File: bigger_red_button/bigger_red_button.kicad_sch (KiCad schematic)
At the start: 22 parts, among them J1 USB_C_Receptacle_USB2.0_16P, J2 Conn_02x05_Odd_Even, J3 Conn_02x01, J4 Conn_02x01, U1 USBLC6-2SC6, U2 TPS7A0533PDBV, U3 STM32C071FBPx, U4 PAM2804

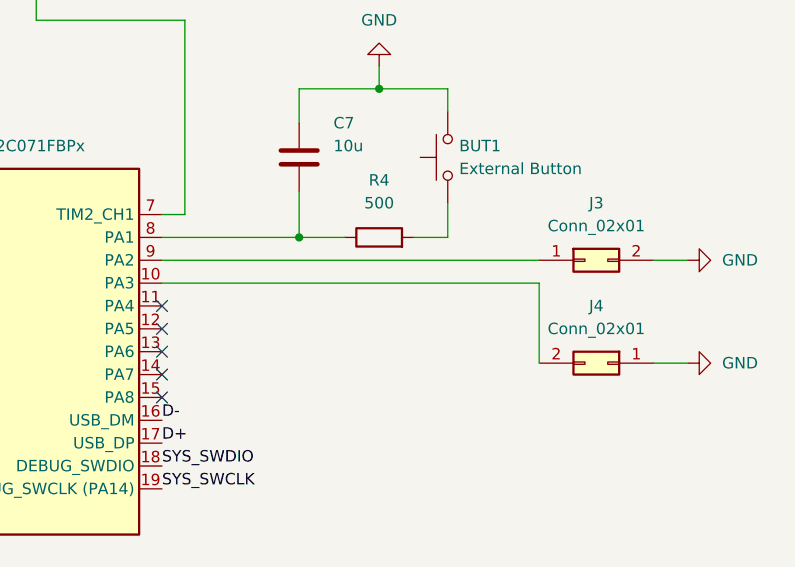
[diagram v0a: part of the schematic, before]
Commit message: Replace jumper symbols
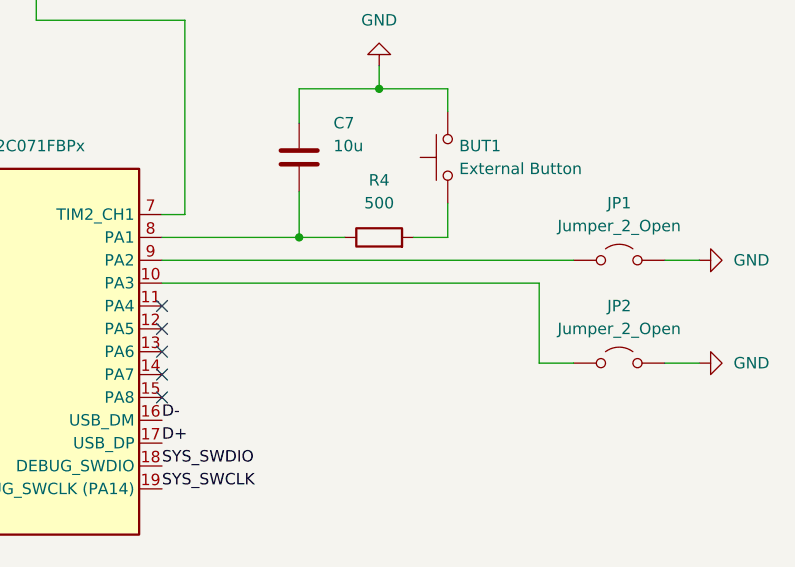
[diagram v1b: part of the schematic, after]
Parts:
- removed J3, J4: Conn_02x01, Connector_PinHeader_2.54mm:PinHeader_1x02_P2.54mm_Vertical, symbol Connector_Generic:Conn_02x01
- added JP1, JP2: Jumper_2_Open, Connector_PinHeader_2.54mm:PinHeader_1x02_P2.54mm_Vertical, symbol Jumper:Jumper_2_Open
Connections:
- net GND: now also JP1.2 (B), JP2.2 (B)
- net at U3.10 (PA3): now also JP2.1 (A)
- net at U3.9 (PA2): now also JP1.1 (A)
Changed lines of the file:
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@@
 	(wire
 		(pts
-			(xy 252.73 106.68) (xy 256.54 106.68)
+			(xy 254 106.68) (xy 257.81 106.68)
 		)
 		(stroke
@@
 	(wire
 		(pts
+			(xy 240.03 118.11) (xy 243.84 118.11)
+		)
+		(stroke
+			(width 0)
+			(type default)
+		)
+	)
+	(wire
+		(pts
 			(xy 213.36 99.06) (xy 213.36 104.14)
 		)
@@
 	(wire
 		(pts
-			(xy 198.12 106.68) (xy 240.03 106.68)
+			(xy 198.12 106.68) (xy 243.84 106.68)
 		)
 		(stroke
@@
 	(wire
 		(pts
-			(xy 252.73 118.11) (xy 256.54 118.11)
+			(xy 254 118.11) (xy 257.81 118.11)
 		)
 		(stroke
@@
 	)
 	(symbol
+		(lib_id "Jumper:Jumper_2_Open")
+		(at 248.92 106.68 0)
+		(unit 1)
+		(exclude_from_sim no)
+		(in_bom yes)
+		(on_board yes)
+		(dnp no)
+		(fields_autoplaced yes)
+		(property "Reference" "JP1"
+			(at 248.92 100.33 0)
+			(effects
+				(font
+					(size 1.27 1.27)
+				)
+			)
+		)
+		(property "Value" "Jumper_2_Open"
+			(at 248.92 102.87 0)
+			(effects
+				(font
+					(size 1.27 1.27)
+				)
+			)
+		)
+		(property "Footprint" "Connector_PinHeader_2.54mm:PinHeader_1x02_P2.54mm_Vertical"
+			(at 248.92 106.68 0)
+			(effects
+				(font
+					(size 1.27 1.27)
+				)
+				(hide yes)
+			)
+		)
+		(property "Datasheet" "~"
+			(at 248.92 106.68 0)
+			(effects
+				(font
+					(size 1.27 1.27)
+				)
+				(hide yes)
+			)
+		)
+		(property "Description" "Jumper, 2-pole, open"
+			(at 248.92 106.68 0)
+			(effects
+				(font
+					(size 1.27 1.27)
+				)
+				(hide yes)
+			)
+		)
+		(pin "2"
+		)
+		(pin "1"
+		)
+		(instances
+			(project ""
+				(path "/feb3b749-4f34-4ca1-ab65-70106c7bdece"
+					(reference "JP1")
+					(unit 1)
+				)
+			)
+		)
+	)
+	(symbol
 		(lib_id "Device:C")
 		(at 100.33 114.3 0)
@@
 	(symbol
 		(lib_id "power:GND")
-		(at 256.54 118.11 90)
+		(at 257.81 118.11 90)
 		(unit 1)
 		(exclude_from_sim no)
@@
 		(fields_autoplaced yes)
 		(property "Reference" "#PWR017"
-			(at 262.89 118.11 0)
+			(at 264.16 118.11 0)
 			(effects
 				(font
@@
 		)
 		(property "Value" "GND"
-			(at 260.35 118.1099 90)
+			(at 261.62 118.1099 90)
 			(effects
 				(font
@@
 		)
 		(property "Footprint" ""
-			(at 256.54 118.11 0)
+			(at 257.81 118.11 0)
 			(effects
 				(font
@@
 		)
 		(property "Datasheet" ""
-			(at 256.54 118.11 0)
+			(at 257.81 118.11 0)
 			(effects
 				(font
@@
 		)
 		(property "Description" "Power symbol creates a global label with name \"GND\" , ground"
-			(at 256.54 118.11 0)
+			(at 257.81 118.11 0)
 			(effects
 				(font
@@
 	)
 	(symbol
-		(lib_id "Connector_Generic:Conn_02x01")
-		(at 245.11 106.68 0)
-		(unit 1)
-		(exclude_from_sim no)
-		(in_bom no)
-		(on_board yes)
-		(dnp no)
-		(fields_autoplaced yes)
-		(property "Reference" "J3"
-			(at 246.38 100.33 0)
-			(effects
-				(font
-					(size 1.27 1.27)
-				)
-			)
-		)
-		(property "Value" "Conn_02x01"
-			(at 246.38 102.87 0)
-			(effects
-				(font
-					(size 1.27 1.27)
-				)
-			)
-		)
-		(property "Footprint" "Connector_PinHeader_2.54mm:PinHeader_1x02_P2.54mm_Vertical"
-			(at 245.11 106.68 0)
-			(effects
-				(font
-					(size 1.27 1.27)
-				)
-				(hide yes)
-			)
-		)
-		(property "Datasheet" "~"
-			(at 245.11 106.68 0)
-			(effects
-				(font
-					(size 1.27 1.27)
-				)
-				(hide yes)
-			)
-		)
-		(property "Description" "Generic connector, double row, 02x01, this symbol is compatible with counter-clockwise, top-bottom and odd-even numbering schemes., script generated (kicad-library-utils/schlib/autogen/connector/)"
-			(at 245.11 106.68 0)
-			(effects
-				(font
-					(size 1.27 1.27)
-				)
-				(hide yes)
-			)
-		)
-		(pin "1"
-		)
-		(pin "2"
-		)
-		(instances
-			(project ""
-				(path "/feb3b749-4f34-4ca1-ab65-70106c7bdece"
-					(reference "J3")
-					(unit 1)
-				)
-			)
-		)
-	)
-	(symbol
 		(lib_id "Device:C")
 		(at 213.36 95.25 0)
@@
 	(symbol
 		(lib_id "power:GND")
-		(at 256.54 106.68 90)
+		(at 257.81 106.68 90)
 		(unit 1)
 		(exclude_from_sim no)
@@
 		(fields_autoplaced yes)
 		(property "Reference" "#PWR016"
-			(at 262.89 106.68 0)
+			(at 264.16 106.68 0)
 			(effects
 				(font
@@
 		)
 		(property "Value" "GND"
-			(at 260.35 106.6799 90)
+			(at 261.62 106.6799 90)
 			(effects
 				(font
@@
 		)
 		(property "Footprint" ""
-			(at 256.54 106.68 0)
+			(at 257.81 106.68 0)
 			(effects
 				(font
@@
 		)
 		(property "Datasheet" ""
-			(at 256.54 106.68 0)
+			(at 257.81 106.68 0)
 			(effects
 				(font
@@
 		)
 		(property "Description" "Power symbol creates a global label with name \"GND\" , ground"
-			(at 256.54 106.68 0)
+			(at 257.81 106.68 0)
 			(effects
 				(font
@@
 	)
 	(symbol
-		(lib_id "Connector_Generic:Conn_02x01")
-		(at 247.65 118.11 0)
-		(mirror y)
+		(lib_id "power:GND")
+		(at 125.73 120.65 0)
 		(unit 1)
 		(exclude_from_sim no)
-		(in_bom no)
+		(in_bom yes)
 		(on_board yes)
 		(dnp no)
-		(property "Reference" "J4"
-			(at 246.38 111.76 0)
+		(fields_autoplaced yes)
+		(property "Reference" "#PWR06"
+			(at 125.73 127 0)
 			(effects
 				(font
 					(size 1.27 1.27)
 				)
+				(hide yes)
 			)
 		)
-		(property "Value" "Conn_02x01"
-			(at 246.38 114.3 0)
+		(property "Value" "GND"
+			(at 125.73 125.73 0)
 			(effects
 				(font
@@
 			)
 		)
-		(property "Footprint" "Connector_PinHeader_2.54mm:PinHeader_1x02_P2.54mm_Vertical"
-			(at 247.65 118.11 0)
+		(property "Footprint" ""
+			(at 125.73 120.65 0)
 			(effects
 				(font
@@
 			)
 		)
-		(property "Datasheet" "~"
-			(at 247.65 118.11 0)
+		(property "Datasheet" ""
+			(at 125.73 120.65 0)
 			(effects
 				(font
@@
 			)
 		)
-		(property "Description" "Generic connector, double row, 02x01, this symbol is compatible with counter-clockwise, top-bottom and odd-even numbering schemes., script generated (kicad-library-utils/schlib/autogen/connector/)"
-			(at 247.65 118.11 0)
+		(property "Description" "Power symbol creates a global label with name \"GND\" , ground"
+			(at 125.73 120.65 0)
 			(effects
 				(font
@@
 			)
 		)
-		(pin "2"
-		)
 		(pin "1"
 		)
@@
 			(project ""
 				(path "/feb3b749-4f34-4ca1-ab65-70106c7bdece"
-					(reference "J4")
+					(reference "#PWR06")
 					(unit 1)
 				)
@@
 	)
 	(symbol
-		(lib_id "power:GND")
-		(at 125.73 120.65 0)
+		(lib_id "Jumper:Jumper_2_Open")
+		(at 248.92 118.11 0)
 		(unit 1)
 		(exclude_from_sim no)
@@
 		(dnp no)
 		(fields_autoplaced yes)
-		(property "Reference" "#PWR06"
-			(at 125.73 127 0)
+		(property "Reference" "JP2"
+			(at 248.92 111.76 0)
 			(effects
 				(font
 					(size 1.27 1.27)
 				)
-				(hide yes)
 			)
 		)
-		(property "Value" "GND"
-			(at 125.73 125.73 0)
+		(property "Value" "Jumper_2_Open"
+			(at 248.92 114.3 0)
 			(effects
 				(font
@@
 			)
 		)
-		(property "Footprint" ""
-			(at 125.73 120.65 0)
+		(property "Footprint" "Connector_PinHeader_2.54mm:PinHeader_1x02_P2.54mm_Vertical"
+			(at 248.92 118.11 0)
 			(effects
 				(font
@@
 			)
 		)
-		(property "Datasheet" ""
-			(at 125.73 120.65 0)
+		(property "Datasheet" "~"
+			(at 248.92 118.11 0)
 			(effects
 				(font
@@
 			)
 		)
-		(property "Description" "Power symbol creates a global label with name \"GND\" , ground"
-			(at 125.73 120.65 0)
+		(property "Description" "Jumper, 2-pole, open"
+			(at 248.92 118.11 0)
 			(effects
 				(font
@@
 		(pin "1"
 		)
+		(pin "2"
+		)
 		(instances
 			(project ""
 				(path "/feb3b749-4f34-4ca1-ab65-70106c7bdece"
-					(reference "#PWR06")
+					(reference "JP2")
 					(unit 1)
 				)
